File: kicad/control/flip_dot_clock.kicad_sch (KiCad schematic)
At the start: 36 parts, among them J1 Conn_01x02_Male, J2 Conn_02x08_Odd_Even, J3 Conn_01x05_Male, U1 NUCLEO-F303K8-HEADER, U10 Small_7_Seg_FlipDot_Module, U2 SLC03B-05, U3 NCV7719, U4 Small_7_Seg_FlipDot_Module, U5 NCV7719, U6 Small_7_Seg_FlipDot_Module, U7 NCV7719, U8 Small_7_Seg_FlipDot_Module, U9 NCV7719

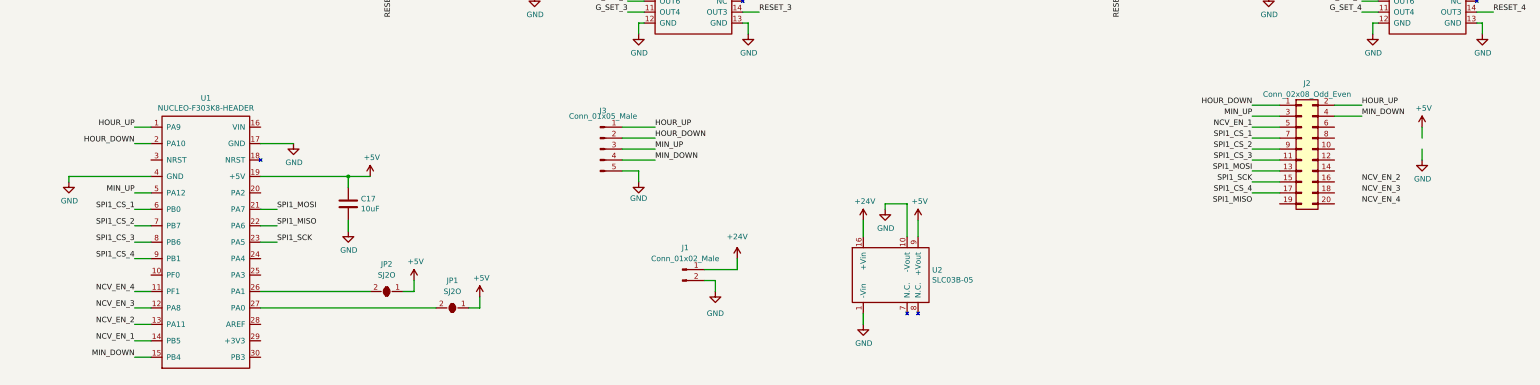
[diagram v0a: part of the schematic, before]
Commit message: moving along
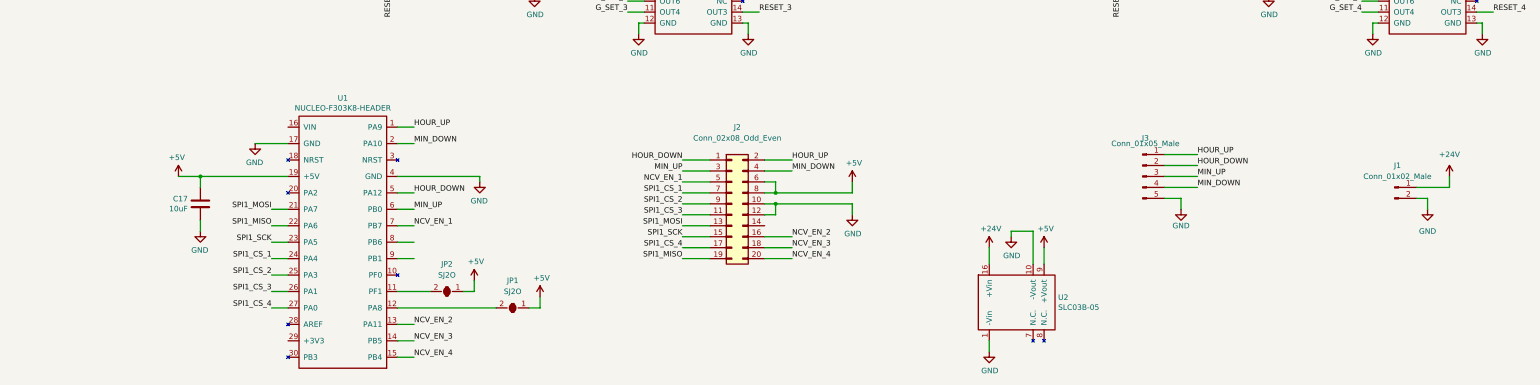
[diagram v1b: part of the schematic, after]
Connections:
- net +5V: now also J2.6 (Pin_6), J2.8 (Pin_8)
- net GND: now also J2.10 (Pin_10), J2.12 (Pin_12)
- net HOUR_DOWN: now also U1.5 (PA12); no longer U1.2 (PA10)
- net MIN_DOWN: now also U1.2 (PA10); no longer U1.15 (PB4)
- net MIN_UP: now also U1.6 (PB0); no longer U1.5 (PA12)
- net NCV_EN_1: now also U1.7 (PB7); no longer U1.14 (PB5)
- net NCV_EN_2: now also J2.16 (Pin_16)
- net NCV_EN_3: now also J2.18 (Pin_18), U1.14 (PB5); no longer U1.12 (PA8)
- net NCV_EN_4: now also J2.20 (Pin_20), U1.15 (PB4); no longer U1.11 (PF1)
- net SPI1_CS_1: now also U1.24 (PA4); no longer U1.6 (PB0)
- net SPI1_CS_2: now also U1.25 (PA3); no longer U1.7 (PB7)
- net SPI1_CS_3: now also U1.26 (PA1); no longer U1.8 (PB6)
- net SPI1_CS_4: now also U1.27 (PA0); no longer U1.9 (PB1)
- net SPI1_MISO: now also J2.19 (Pin_19)
- net at JP2.2 (B): now also U1.11 (PF1); no longer U1.26 (PA1)
- net at JP1.2 (B): now also U1.12 (PA8); no longer U1.27 (PA0)
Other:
- moved on the sheet: C17, J1, J2, J3, JP1, JP2, U2
